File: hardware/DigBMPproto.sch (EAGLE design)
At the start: 30 parts, among them IC1 INA126U, IC3 OPA4344U, IC4 OPA4344U, IC5 OPA4344U

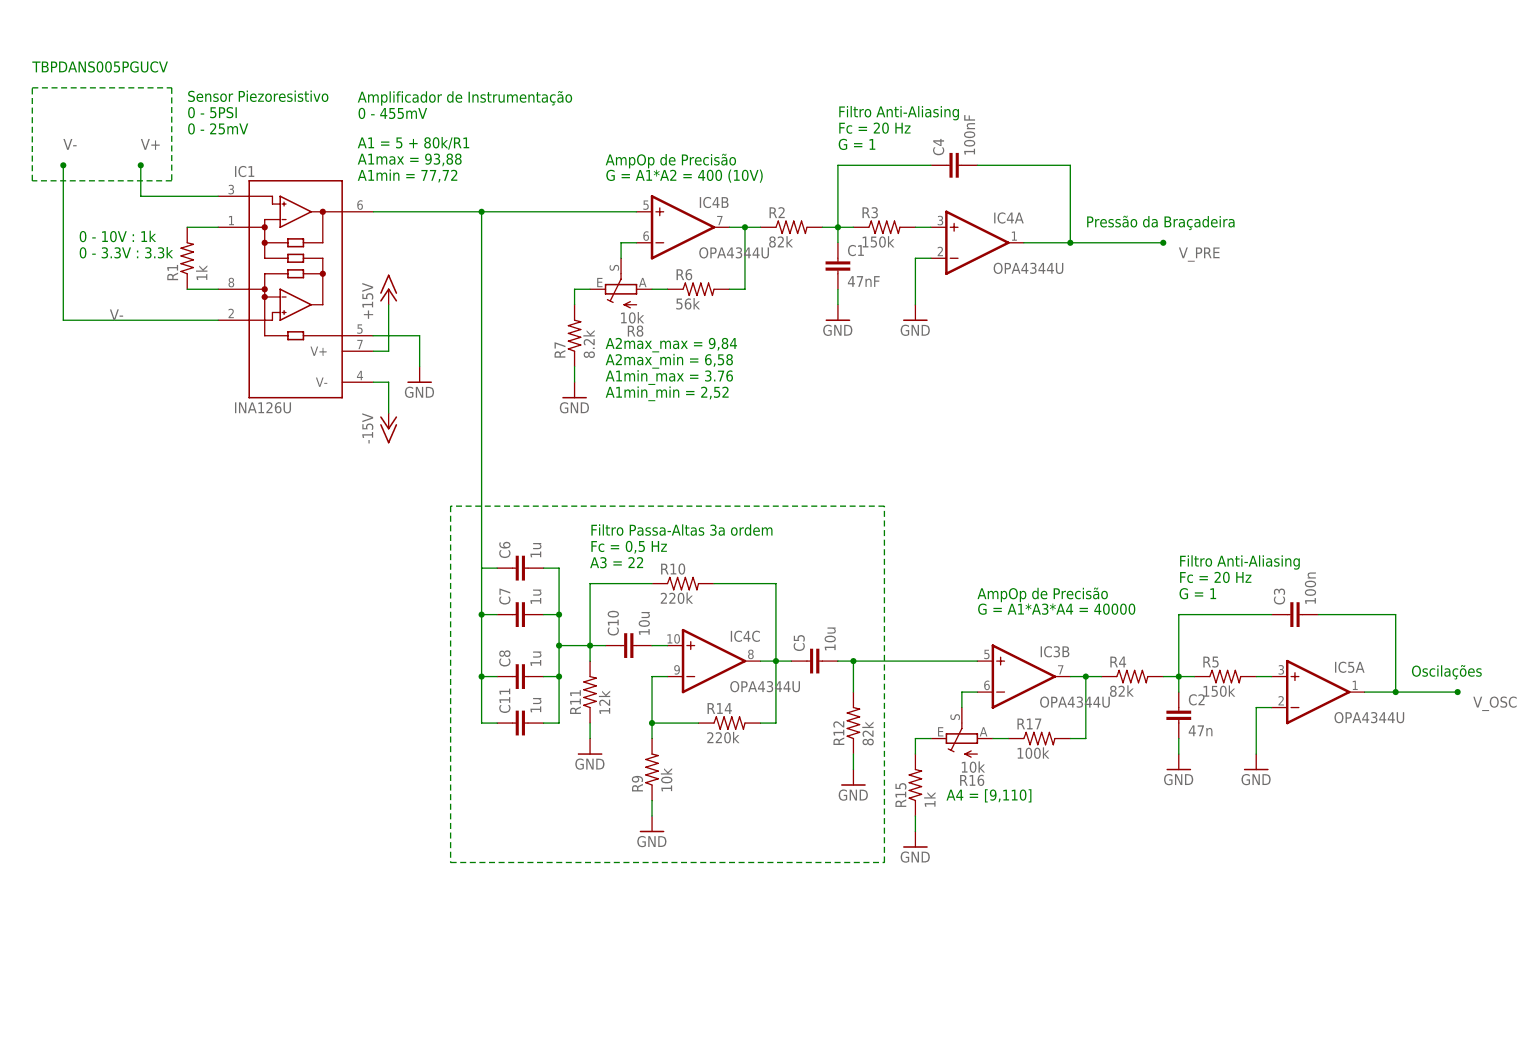
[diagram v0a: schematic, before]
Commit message: Eagle Schematic
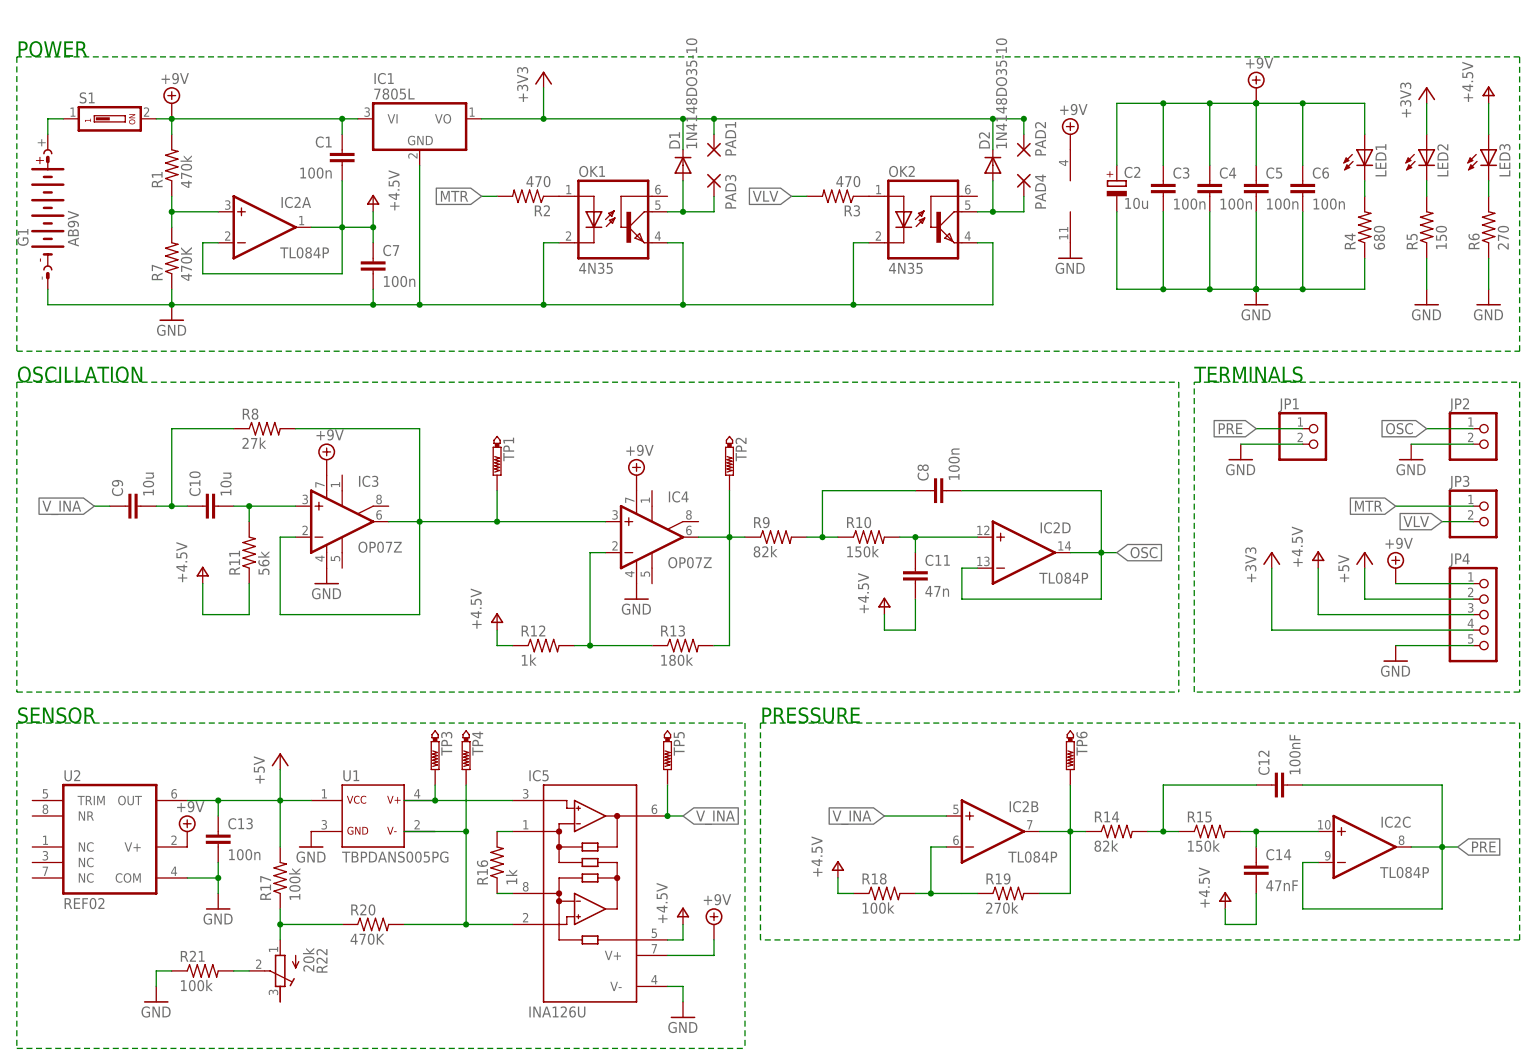
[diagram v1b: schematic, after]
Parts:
- added C12: 100nF, rcl:C-EUC3216
- added C13: 100n, rcl:C-EU050-025X075
- added C14: 47nF, rcl:C-EUC3216
- added C9: 10u, rcl:C-EUC3216
- added D1, D2: 1N4148DO35-10, diode:1N4148DO35-10
- added G1: AB9V, battery:AB9V
- added IC2: TL084P, linear:TL084P
- added JP1, JP2, JP3: (no value), pinhead:PINHD-1X2
- added JP4: (no value), pinhead:PINHD-1X5
- added LED1, LED2, LED3: (no value), led:LED3MM
- added OK1, OK2: 4N35, optocoupler:4N35
- added PAD1, PAD2, PAD3, PAD4: (no value), wirepad:1,6/0,8
- added R13: 180k, rcl:R-US_0207/7
- added R18, R21: 100k, rcl:R-US_0207/7
- added R19: 270k, rcl:R-US_0207/7
- added R20: 470K, rcl:R-US_0207/7
- added R22: 20k, rcl:R-TRIMM64W
- added S1: (no value), switch-dil:DS01
- added TP1, TP2, TP3, TP4, TP5, TP6: PTR1PAD1-13, testpad:PTR1PAD1-13
- added U1: TBPDANS005PG, honeywell:TBPDANS005PG
- added U2: REF02, custom:REF02
- C1: value 47nF -> 100n; device rcl:C-EUC3216 -> rcl:C-EU050-025X075
- C11: value 1u -> 47n
- C2: value 47n -> 10u; device rcl:C-EUC3216 -> rcl:CPOL-EUE2.5-5
- C3: device rcl:C-EUC3216 -> rcl:C-EU050-025X075
- C4: value 100nF -> 100n; device rcl:C-EUC3216 -> rcl:C-EU050-025X075
- C5: value 10u -> 100n; device rcl:C-EUC3216 -> rcl:C-EU050-025X075
- C6, C7: value 1u -> 100n; device rcl:C-EUC3216 -> rcl:C-EU050-025X075
- C8: value 1u -> 100n
- IC1: value INA126U -> 7805L; device burr-brown:INA126U -> linear:7805L
- IC3, IC4: value OPA4344U -> OP07Z; device linear:OPA4344U -> linear:OP07Z
- IC5: value OPA4344U -> INA126U; device linear:OPA4344U -> burr-brown:INA126U
- R1: value 1k -> 470k; device resistor:R-US_M1206 -> rcl:R-US_0207/7
- R10: value 220k -> 150k; device resistor:R-US_M1206 -> rcl:R-US_0207/7
- R11: value 12k -> 56k; device resistor:R-US_M1206 -> rcl:R-US_0207/7
- R12: value 82k -> 1k; device resistor:R-US_M1206 -> rcl:R-US_0207/7
- R14: value 220k -> 82k; device resistor:R-US_M1206 -> rcl:R-US_0207/7
- R15: value 1k -> 150k; device resistor:R-US_M1206 -> rcl:R-US_0207/7
- R16: value 10k -> 1k; device pot:TRIM_EU-B64Y -> resistor:R-US_M1206
- R17: device resistor:R-US_M1206 -> rcl:R-US_0207/7
- R2: value 82k -> 470; device resistor:R-US_M1206 -> rcl:R-US_0207/7
- R3: value 150k -> 470; device resistor:R-US_M1206 -> rcl:R-US_0207/7
- R4: value 82k -> 680; device resistor:R-US_M1206 -> rcl:R-US_0207/7
- R5: value 150k -> 150; device resistor:R-US_M1206 -> rcl:R-US_0207/7
- R6: value 56k -> 270; device resistor:R-US_M1206 -> rcl:R-US_0207/7
- R7: value 8.2k -> 470K; device resistor:R-US_M1206 -> rcl:R-US_0207/7
- R8: value 10k -> 27k; device pot:TRIM_EU-B64Y -> rcl:R-US_0207/7
- R9: value 10k -> 82k; device resistor:R-US_M1206 -> rcl:R-US_0207/7
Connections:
- removed net N$13: C3.2, IC5A.OUT
- removed net N$22: R16.A, R17.1
- removed net N$7: C5.2, IC3B.+IN, R12.2
- removed net V1: C11.1, C6.1, C7.1, C8.1, IC1.OUT, IC4B.+IN
- removed net V_PRE: C4.2, IC4A.OUT
- new net +3V3: D1.C, D2.C, IC1.VO, JP4.4, LED2.A, PAD1.P, PAD2.P
- new net +5V: JP4.2
- new net +9V: C1.1, C2.+, C3.1, C4.1, C5.1, C6.1, IC1.VI, IC2P.V+, IC3.V+, IC4.V+, IC5.V+, JP4.1, LED1.A, R1.2, S1.2, U2.V+
- new net MTR: JP3.1, R2.2
- new net N$1: IC2A.+IN, R1.1, R7.2
- new net N$15: D2.A, OK2.COL, PAD4.P
- new net N$23: G1.+, S1.1
- new net N$24: OK2.A, R3.1
- new net N$25: OK1.A, R2.1
- new net N$26: R17.1, R20.1, R22.A
- new net N$27: LED3.C, R6.2
- new net N$30: R21.2, R22.S
- new net OSC: C8.2, IC2D.-IN, IC2D.OUT, JP2.1
- new net PRE: C12.2, IC2C.-IN, IC2C.OUT, JP1.1
- new net VCC: C13.1, R17.2, U1.VCC, U2.OUT
- new net VLV: JP3.2, R3.2
- new net V_INA: C9.1, IC2B.+IN, IC5.OUT, TP5.TP
- net GND: now also C13.2, C2.-, C3.2, C4.2, C5.2, C6.2, C7.2, G1.-, IC1.GND, IC2P.V-, IC3.V-, IC4.V-, IC5.V-, JP1.2, JP2.2, JP4.5, OK1.C, OK1.EMI, OK2.C, OK2.EMI, R21.1, R4.1, R5.1, R6.1, U1.GND, U2.COM; no longer C1.2, C2.2, IC1.REF, IC4A.-IN, IC5A.-IN, R11.1, R12.1, R15.1, R9.1
- net N$10: now also C8.1, R10.1, R9.2; no longer C2.1, C3.1, R4.2, R5.1
- net N$11: now also IC2B.-IN, R18.2; no longer R7.2, R8.E
- net N$12: now also D1.A, OK1.COL, PAD3.P; no longer IC4B.-IN, R8.S
- net N$14: now also R19.1; no longer R6.1, R8.A
- net N$16: now also IC3.-IN, IC3.OUT, IC4.+IN, R8.2, TP1.TP; no longer IC4C.-IN, R14.1, R9.2
- net N$17: now also C9.2, R8.1; no longer C11.2, C6.2, C7.2, C8.2, R10.1, R11.2
- net N$18: now also LED2.C, R5.2; no longer C5.1, IC4C.OUT, R10.2, R14.2
- net N$19: now also IC4.-IN, R12.2, R13.1; no longer R15.2, R16.E
- net N$2: now also IC2B.OUT, R14.1, R19.2, TP6.TP; no longer IC4B.OUT, R2.1, R6.2
- net N$20: now also C11.1, IC2D.+IN, R10.2; no longer IC5A.+IN, R5.2
- net N$21: now also LED1.C, R4.2; no longer IC3B.-IN, R16.S
- net N$3: now also IC5.RG, R16.2; no longer IC1.RG, R1.2
- net N$4: now also IC5.RG@1, R16.1; no longer IC1.RG@1, R1.1
- net N$5: now also C14.1, IC2C.+IN, R15.2; no longer IC4A.+IN, R3.2
- net N$6: now also C12.1, R14.2, R15.1; no longer C1.1, C4.1, R2.2, R3.1
- net N$8: now also IC4.OUT, R13.2, R9.1, TP2.TP; no longer IC3B.OUT, R17.2, R4.1
- net N$9: now also IC3.+IN, R11.2; no longer IC4C.+IN
- net V+: now also C1.2, C11.2, C14.2, C7.1, IC2A.-IN, IC2A.OUT, IC5.+IN, IC5.REF, JP4.3, LED3.A, R11.1, R12.1, R18.1, TP3.TP, U1.V+; no longer IC1.+IN
- net V-: now also IC5.-IN, R20.2, TP4.TP, U1.V-; no longer IC1.-IN
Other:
- note added: "OSCILLATION"
- note added: "POWER"
- note added: "PRESSURE"
- note added: "SENSOR"
- note added: "TERMINALS"
- note removed: "0 - 10V : 1k 0 - 3.3V : 3.3k"
- note removed: "A1 = 5 + 80k/R1 A1max = 93,88 A1min = 77,72"
- note removed: "A2max_max = 9,84 A2max_min = 6,58 A1min_max = 3.76 A1min_min = 2,52"
- note removed: "A4 = [9,110]"
- note removed: "AmpOp de Precisão"
- note removed: "Amplificador de Instrumentação 0 - 455mV"
- note removed: "Filtro Anti-Aliasing Fc = 20 Hz G = 1"
- note removed: "Filtro Passa-Altas 3a ordem Fc = 0,5 Hz A3 = 22"
- note removed: "G = A1*A2 = 400 (10V)"
- note removed: "G = A1*A3*A4 = 40000"
- note removed: "Oscilações"
- note removed: "Pressão da Braçadeira"
- note removed: "Sensor Piezoresistivo 0 - 5PSI 0 - 25mV"
- note removed: "TBPDANS005PGUCV"
- moved on the sheet: C1, C10, C11, C3, C4, C5, C6, C7, C8, R1, R10, R11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
